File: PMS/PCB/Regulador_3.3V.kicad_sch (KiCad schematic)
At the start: 16 parts, among them U7 MP1584

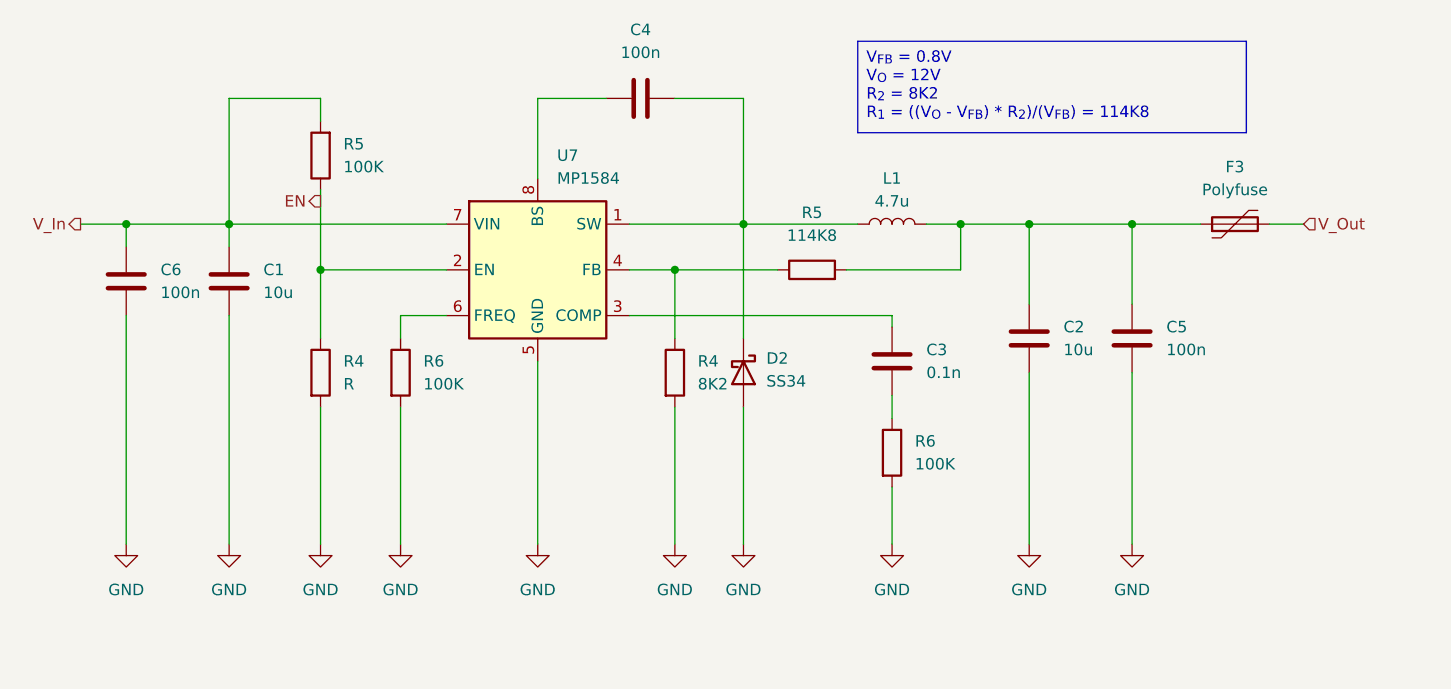
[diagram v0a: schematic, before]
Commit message: Continua Desarrollo
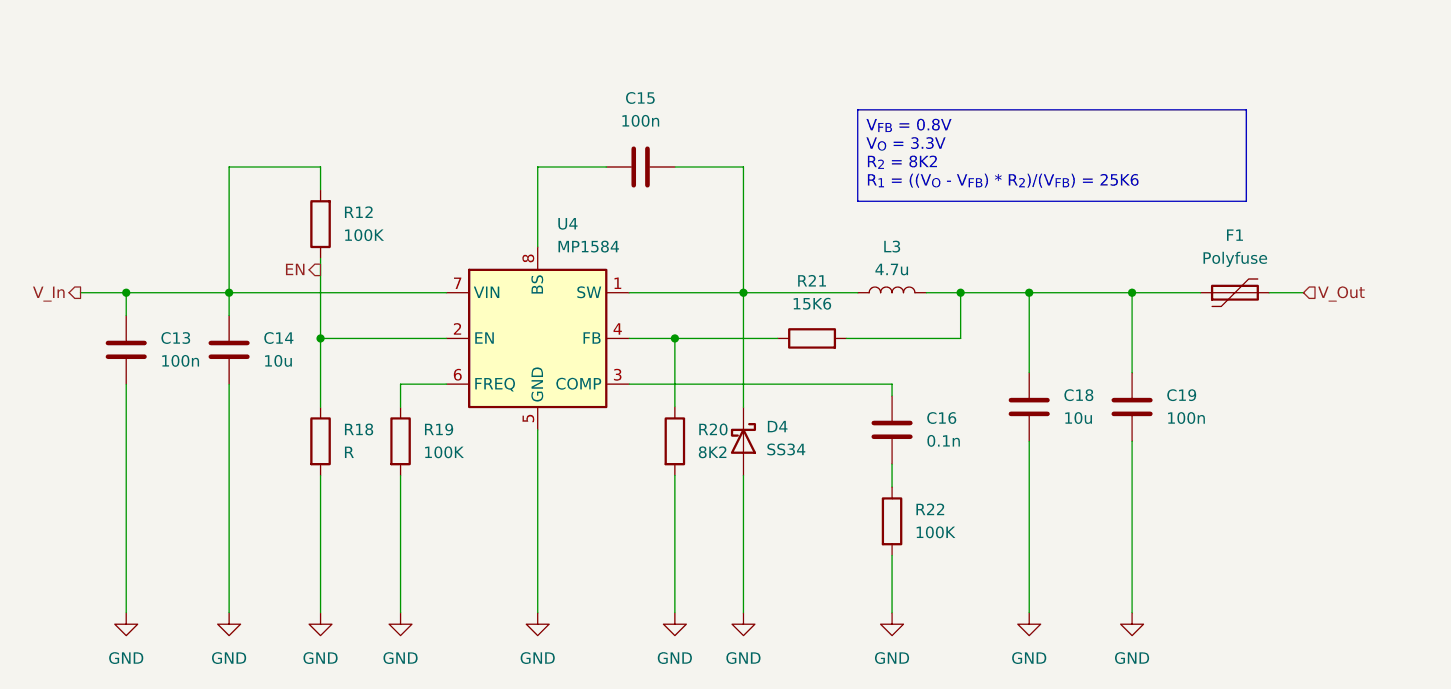
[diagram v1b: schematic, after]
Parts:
- removed C1, C2: 10u, symbol Device:C
- removed C3: 0.1n, symbol Device:C
- removed C4, C5, C6: 100n, symbol Device:C
- removed D2: SS34, symbol Device:D_Schottky
- removed F3: Polyfuse, symbol Device:Polyfuse
- removed L1: 4.7u, symbol Device:L
- removed R4: R, symbol Device:R
- removed R4: 8K2, symbol Device:R
- removed R5, R6 (x2): 100K, symbol Device:R
- removed R5: 114K8, symbol Device:R
- removed U7: MP1584, Package_SO:SOIC-8-1EP_3.9x4.9mm_P1.27mm_EP2.62x3.51mm, symbol CubeSat:MP1584EN
- added C13, C15, C19: 100n, symbol Device:C
- added C14, C18: 10u, symbol Device:C
- added C16: 0.1n, symbol Device:C
- added D4: SS34, symbol Device:D_Schottky
- added F1: Polyfuse, symbol Device:Polyfuse
- added L3: 4.7u, symbol Device:L
- added R12, R19, R22: 100K, symbol Device:R
- added R18: R, symbol Device:R
- added R20: 8K2, symbol Device:R
- added R21: 15K6, symbol Device:R
- added U4: MP1584, Package_SO:SOIC-8-1EP_3.9x4.9mm_P1.27mm_EP2.62x3.51mm, symbol CubeSat:MP1584EN
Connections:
- net EN: now also R12.1, R18.1, U4.2 (EN)
- net GND: now also C13.2, C14.2, C18.2, C19.2, D4.2 (A), R18.2, R19.2, R20.2, R22.2, U4.5 (GND)
- net V_In: now also C13.1, C14.1, R12.2, U4.7 (VIN)
- net V_Out: now also F1.2
- new net: C16.1, U4.3 (COMP)
- new net: C16.2, R22.1
- new net: C15.2, D4.1 (K), L3.1, U4.1 (SW)
- new net: C18.1, C19.1, F1.1, L3.2, R21.2
- new net: R20.1, R21.1, U4.4 (FB)
- new net: R19.1, U4.6 (FREQ)
- new net: C15.1, U4.8 (BS)
